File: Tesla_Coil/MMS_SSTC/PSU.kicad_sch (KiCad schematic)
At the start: 3 parts, among them U6 TL494IN, U7 TL071CP

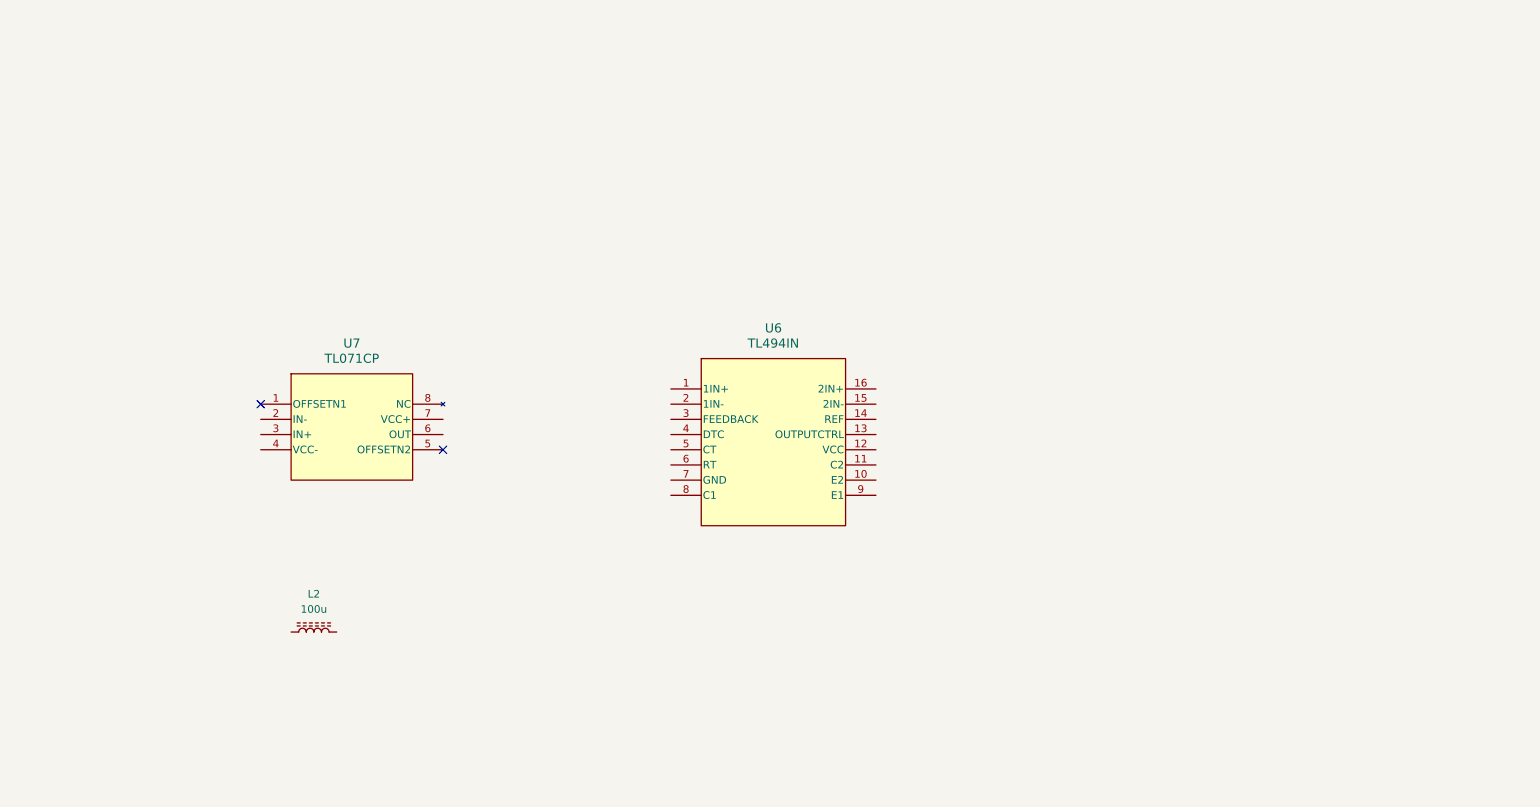
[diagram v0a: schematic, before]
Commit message: Commit additions to SSTC PSU schematic
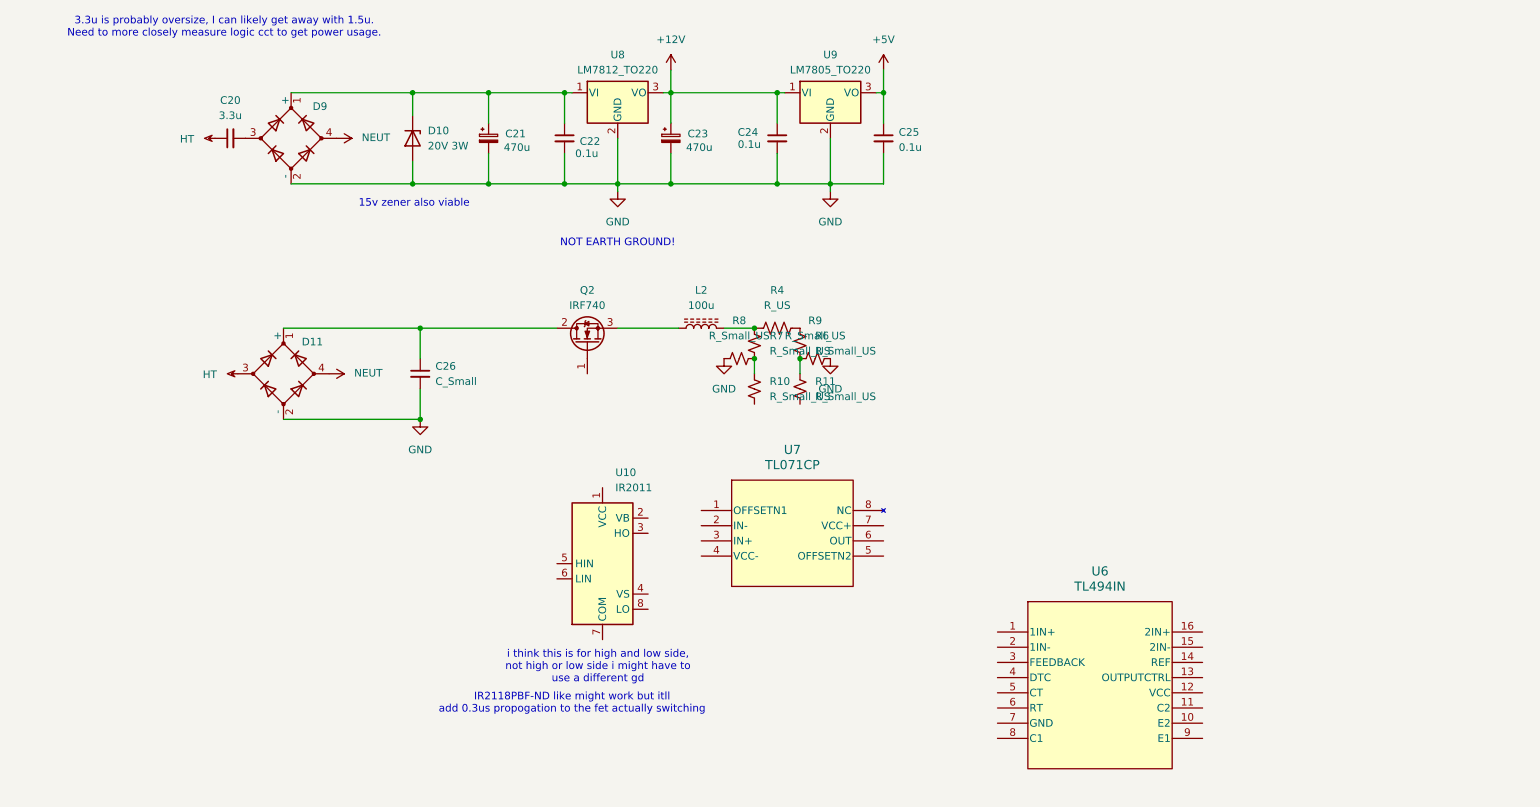
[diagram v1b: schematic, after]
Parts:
- added C20: 3.3u, Capacitor_THT:C_Rect_L31.5mm_W17.0mm_P27.50mm_MKS4, symbol Device:C_Small
- added C21, C23: 470u, Capacitor_THT:CP_Radial_D12.5mm_P5.00mm, symbol Device:C_Polarized_Small
- added C22, C24, C25: 0.1u, Capacitor_THT:C_Disc_D3.0mm_W2.0mm_P2.50mm, symbol Device:C_Small
- added C26: C_Small, symbol Device:C_Small
- added D10: 20V 3W, symbol Device:D_Zener
- added D11, D9: D_Bridge_+-AA, symbol Device:D_Bridge_+-AA
- added Q2: IRF740, Package_TO_SOT_THT:TO-220-3_Vertical, symbol Transistor_FET:IRF740
- added R10, R11, R6, R7, R8, R9: R_Small_US, symbol Device:R_Small_US
- added R4: R_US, symbol Device:R_US
- added U10: IR2011, symbol Driver_FET:IR2011
- added U8: LM7812_TO220, Package_TO_SOT_THT:TO-220-3_Vertical, symbol Regulator_Linear:LM7812_TO220
- added U9: LM7805_TO220, Package_TO_SOT_THT:TO-220-3_Vertical, symbol Regulator_Linear:LM7805_TO220
- U7: DKPN (none) -> 296-7186-5-ND
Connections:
- net at L2.1: now also Q2.3 (S)
- net at L2.2: now also R4.1, R7.1
- new net: R10.1, R7.2, R8.2
- new net: R11.1, R6.2, R9.1
- new net: C21.1, C22.1, D10.1 (K), D9.1 (+), U8.1 (VI)
- new net: C20.2, D9.3
- new net: R4.2, R6.1
- new net: C26.1, D11.1 (+), Q2.2 (D)
- new net +12V: C23.1, C24.1, U8.3 (VO), U9.1 (VI)
- new net +5V: C25.1, U9.3 (VO)
- new net GND: C21.2, C22.2, C23.2, C24.2, C25.2, C26.2, D10.2 (A), D11.2 (-), D9.2 (-), R8.1, R9.2, U8.2 (GND), U9.2 (GND)
- new net HT: C20.1, D11.3
- new net NEUT: D11.4, D9.4
- no-connect marks 2 -> 0
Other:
- note added: "15v zener also viable"
- note added: "3.3u is probably oversize, I can likely get away with 1.5u. Need to more closely measure logic cct to get power usage."
- note added: "IR2118PBF-ND like might work but itll add 0.3us propogation to the fet actually switching"
- note added: "NOT EARTH GROUND!"
- note added: "i think this is for high and low side, not high or low side i might have to use a different gd"
- moved on the sheet: L2, U6, U7

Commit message: Begin work on final tesla coil design
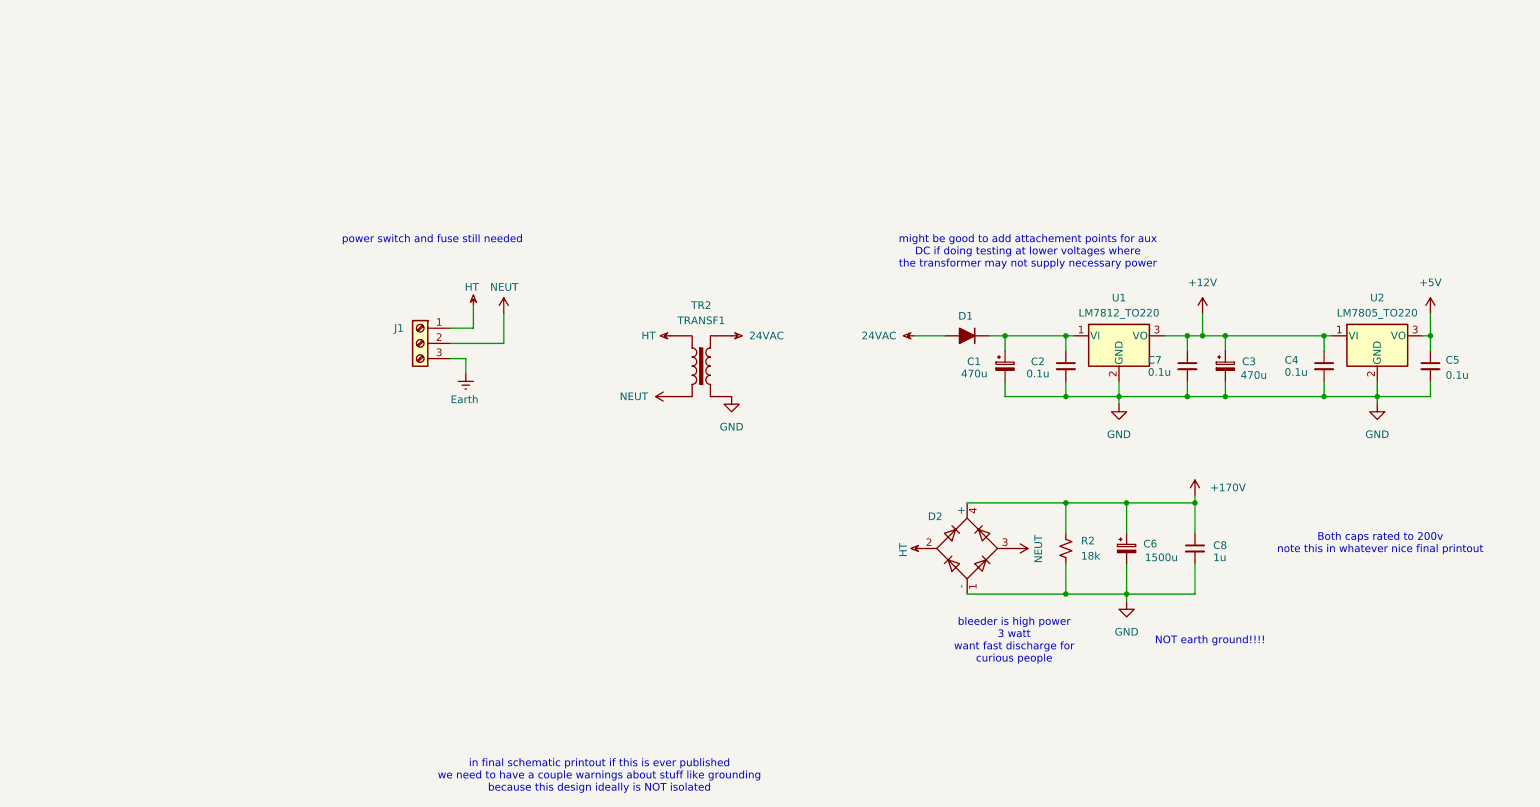
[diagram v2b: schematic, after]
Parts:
- removed C20: 3.3u, Capacitor_THT:C_Rect_L31.5mm_W17.0mm_P27.50mm_MKS4, symbol Device:C_Small
- removed C21, C23: 470u, Capacitor_THT:CP_Radial_D12.5mm_P5.00mm, symbol Device:C_Polarized_Small
- removed C22, C24, C25: 0.1u, Capacitor_THT:C_Disc_D3.0mm_W2.0mm_P2.50mm, symbol Device:C_Small
- removed C26: C_Small, symbol Device:C_Small
- removed D10: 20V 3W, symbol Device:D_Zener
- removed D11, D9: D_Bridge_+-AA, symbol Device:D_Bridge_+-AA
- removed L2: 100u, Inductor_THT:L_Radial_D21.0mm_P19.00mm, symbol Device:L_Ferrite
- removed Q2: IRF740, Package_TO_SOT_THT:TO-220-3_Vertical, symbol Transistor_FET:IRF740
- removed R10, R11, R6, R7, R8, R9: R_Small_US, symbol Device:R_Small_US
- removed R4: R_US, symbol Device:R_US
- removed U10: IR2011, symbol Driver_FET:IR2011
- removed U6: TL494IN, Package_DIP:DIP-16_W7.62mm, symbol locals:TL494IN
- removed U7: TL071CP, Package_DIP:DIP-8_W7.62mm, symbol locals:TL071CP
- removed U8: LM7812_TO220, Package_TO_SOT_THT:TO-220-3_Vertical, symbol Regulator_Linear:LM7812_TO220
- removed U9: LM7805_TO220, Package_TO_SOT_THT:TO-220-3_Vertical, symbol Regulator_Linear:LM7805_TO220
- added C1, C3: 470u, Capacitor_THT:CP_Radial_D12.5mm_P5.00mm, symbol Device:C_Polarized_Small
- added C2, C4, C5, C7: 0.1u, Capacitor_THT:C_Disc_D3.0mm_W2.0mm_P2.50mm, symbol Device:C_Small
- added C6: 1500u, Capacitor_THT:CP_Radial_D30.0mm_P10.00mm_SnapIn, symbol Device:C_Polarized_Small
- added C8: 1u, Capacitor_THT:C_Rect_L18.0mm_W7.0mm_P15.00mm_FKS3_FKP3, symbol Device:C_Small
- added D1: D_Filled, Diode_THT:D_DO-41_SOD81_P7.62mm_Horizontal, symbol Device:D_Filled
- added D2: B125C2300-1500A, Diode_THT:Diode_Bridge_Vishay_GBU, symbol Diode_Bridge:B125C2300-1500A
- added J1: Screw_Terminal_01x02, locals:691137710003, symbol Connector:Screw_Terminal_01x03
- added R2: 18k, Resistor_THT:R_Axial_DIN0617_L17.0mm_D6.0mm_P5.08mm_Vertical, symbol Device:R_Small_US
- added TR2: TRANSF1, symbol Transformer:TRANSF1
- added U1: LM7812_TO220, Package_TO_SOT_THT:TO-220-3_Vertical, symbol Regulator_Linear:LM7812_TO220
- added U2: LM7805_TO220, Package_TO_SOT_THT:TO-220-3_Vertical, symbol Regulator_Linear:LM7805_TO220
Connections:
- net +12V: now also C3.1, C4.1, C7.1, U1.3 (VO), U2.1 (VI)
- net +5V: now also C5.1, U2.3 (VO)
- net GND: now also C1.2, C2.2, C3.2, C4.2, C5.2, C6.2, C7.2, C8.2, D2.1 (-), R2.2, TR2.3, U1.2 (GND), U2.2 (GND)
- net HT: now also D2.2, J1.1 (Pin_1), TR2.1
- net NEUT: now also D2.3, J1.2 (Pin_2), TR2.2
- new net: C1.1, C2.1, D1.1 (K), U1.1 (VI)
- new net +170V: C6.1, C8.1, D2.4 (+), R2.1
- new net 24VAC: D1.2 (A), TR2.4
- new net Earth: J1.3 (Pin_3)
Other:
- note added: "Both caps rated to 200v note this in whatever nice final printout"
- note added: "NOT earth ground!!!!"
- note added: "bleeder is high power 3 watt want fast discharge for curious people"
- note added: "in final schematic printout if this is ever published we need to have a couple warnings about stuff like grounding because this design ideally is NOT isolated"
- note added: "might be good to add attachement points for aux DC if doing testing at lower voltages where the transformer may not supply necessary power"
- note added: "power switch and fuse still needed"
- note removed: "15v zener also viable"
- note removed: "3.3u is probably oversize, I can likely get away with 1.5u. Need to more closely measure logic cct to get power usage."
- note removed: "IR2118PBF-ND like might work but itll add 0.3us propogation to the fet actually switching"
- note removed: "NOT EARTH GROUND!"
- note removed: "i think this is for high and low side, not high or low side i might have to use a different gd"
